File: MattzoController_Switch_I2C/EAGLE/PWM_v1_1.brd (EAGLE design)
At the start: 90 x 90 mm, 10 parts, among them X1 MSTBA2, X4 057-016-0

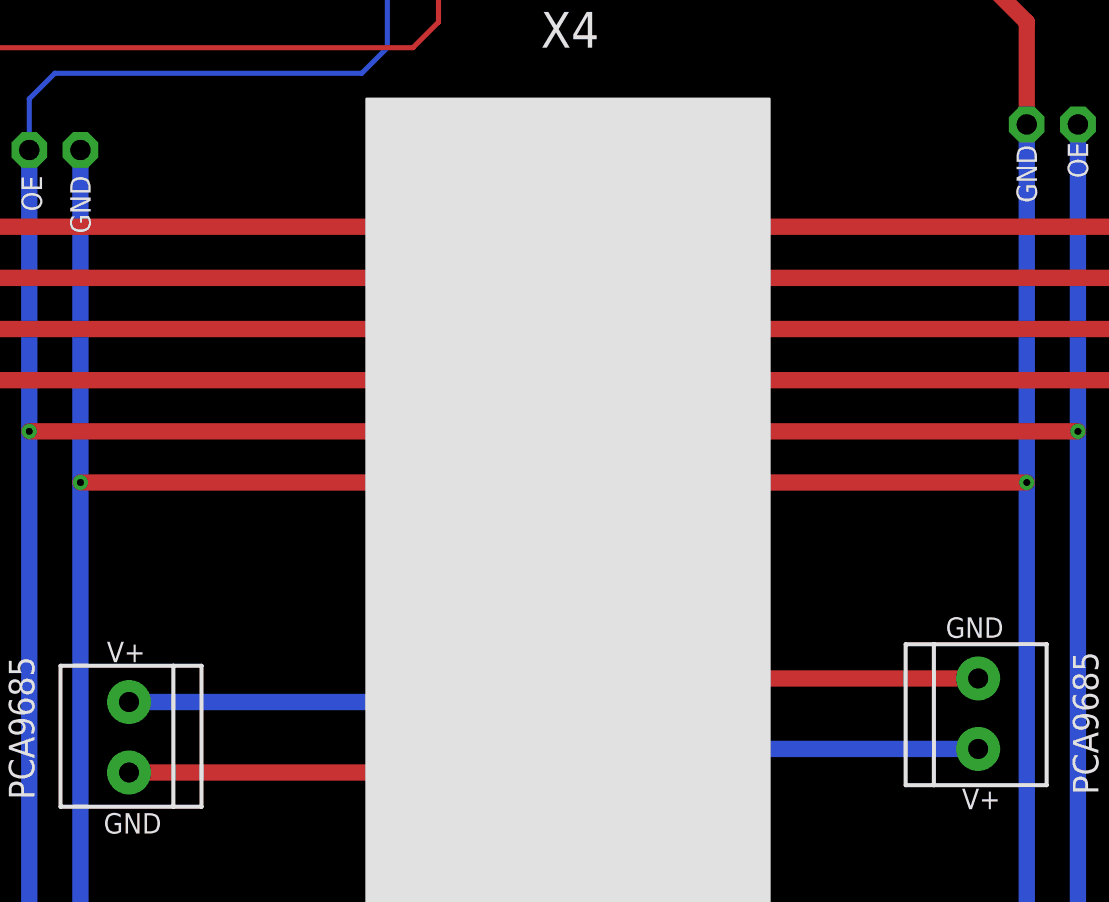
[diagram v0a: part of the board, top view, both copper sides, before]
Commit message: Update PWM_v1_1.brd
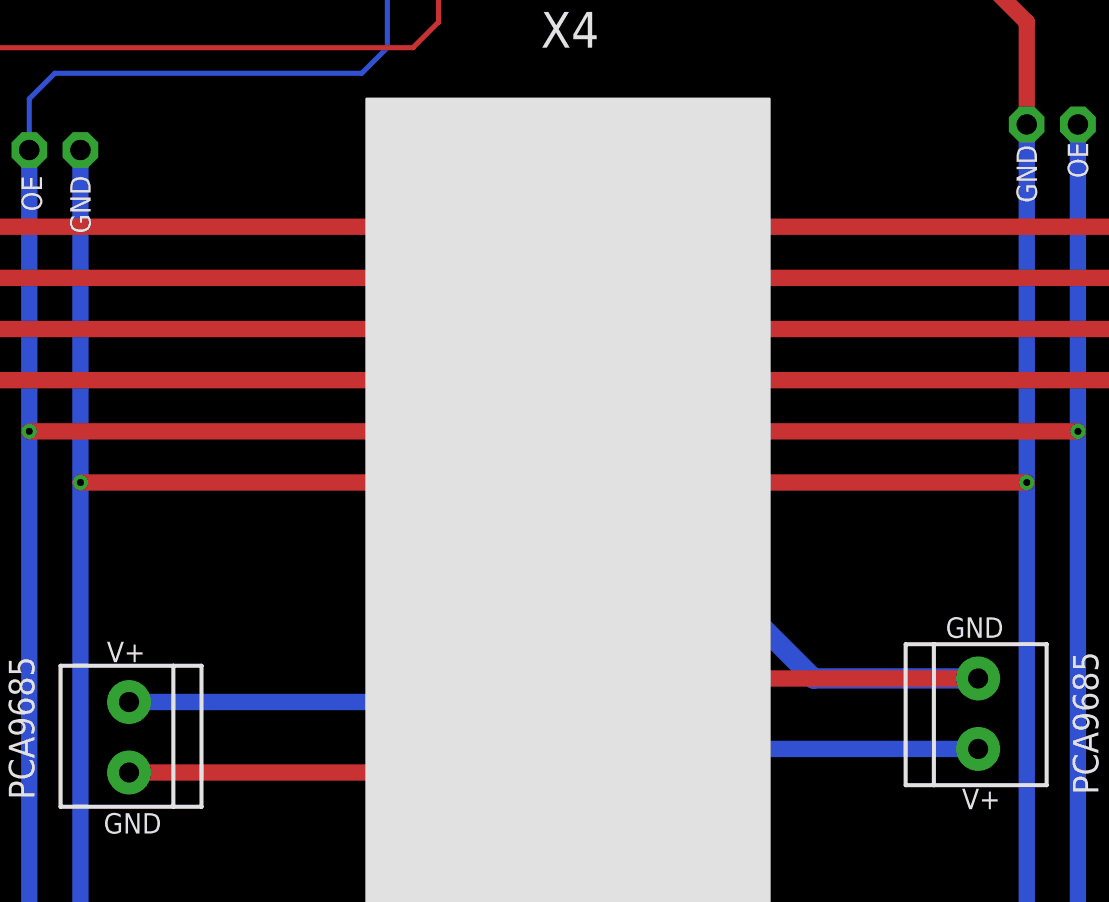
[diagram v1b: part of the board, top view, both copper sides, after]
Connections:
- net N$1: now also U$2.OUT-; no longer U$2.OUT+
- net N$2: now also U$2.OUT+; no longer U$2.OUT-
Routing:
- net N$1: track 76.2 -> 81.0 mm, vias 1 -> 0
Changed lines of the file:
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@@
 <contactref element="J2" pad="2"/>
 <wire x1="66.167" y1="43.61" x2="48.69" y2="43.61" width="0.8128" layer="1"/>
-<wire x1="44.02" y1="38.94" x2="36.83" y2="38.94" width="0.8128" layer="1"/>
-<wire x1="36.83" y1="38.94" x2="24.003" y2="38.94" width="0.8128" layer="1"/>
+<wire x1="44.02" y1="38.94" x2="24.003" y2="38.94" width="0.8128" layer="1"/>
 <wire x1="48.69" y1="43.61" x2="44.02" y2="38.94" width="0.8128" layer="1"/>
-<contactref element="U$2" pad="OUT+"/>
-<wire x1="37.4" y1="70.79" x2="37.4" y2="48.83" width="0.8128" layer="16"/>
-<wire x1="37.4" y1="48.83" x2="36.83" y2="48.26" width="0.8128" layer="16"/>
-<via x="36.83" y="48.26" extent="1-16" drill="0.35"/>
-<wire x1="36.83" y1="48.26" x2="36.83" y2="38.94" width="0.8128" layer="1"/>
+<contactref element="U$2" pad="OUT-"/>
+<wire x1="66.167" y1="43.61" x2="57.99" y2="43.61" width="1.016" layer="16"/>
+<wire x1="54.2" y1="47.4" x2="54.2" y2="70.79" width="1.016" layer="16"/>
+<wire x1="57.99" y1="43.61" x2="54.2" y2="47.4" width="1.016" layer="16"/>
 </signal>
 <signal name="N$2">
 <contactref element="J3" pad="1"/>
 <contactref element="J2" pad="1"/>
-<wire x1="24.003" y1="42.44" x2="45.19" y2="42.44" width="0.8128" layer="16"/>
+<wire x1="24.003" y1="42.44" x2="41.91" y2="42.44" width="0.8128" layer="16"/>
+<wire x1="41.91" y1="42.44" x2="45.19" y2="42.44" width="0.8128" layer="16"/>
 <wire x1="47.52" y1="40.11" x2="54.61" y2="40.11" width="0.8128" layer="16"/>
 <wire x1="54.61" y1="40.11" x2="66.167" y2="40.11" width="0.8128" layer="16"/>
 <wire x1="45.19" y1="42.44" x2="47.52" y2="40.11" width="0.8128" layer="16"/>
-<contactref element="U$2" pad="OUT-"/>
-<wire x1="54.2" y1="70.79" x2="54.2" y2="40.52" width="0.8128" layer="16"/>
 <wire x1="54.2" y1="40.52" x2="54.61" y2="40.11" width="0.8128" layer="16"/>
+<contactref element="U$2" pad="OUT+"/>
+<wire x1="41.91" y1="42.44" x2="37.4" y2="46.95" width="1.016" layer="16"/>
+<wire x1="37.4" y1="46.95" x2="37.4" y2="70.79" width="1.016" layer="16"/>
 </signal>
 <signal name="N$11">
